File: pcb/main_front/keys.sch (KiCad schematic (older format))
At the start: 303 parts

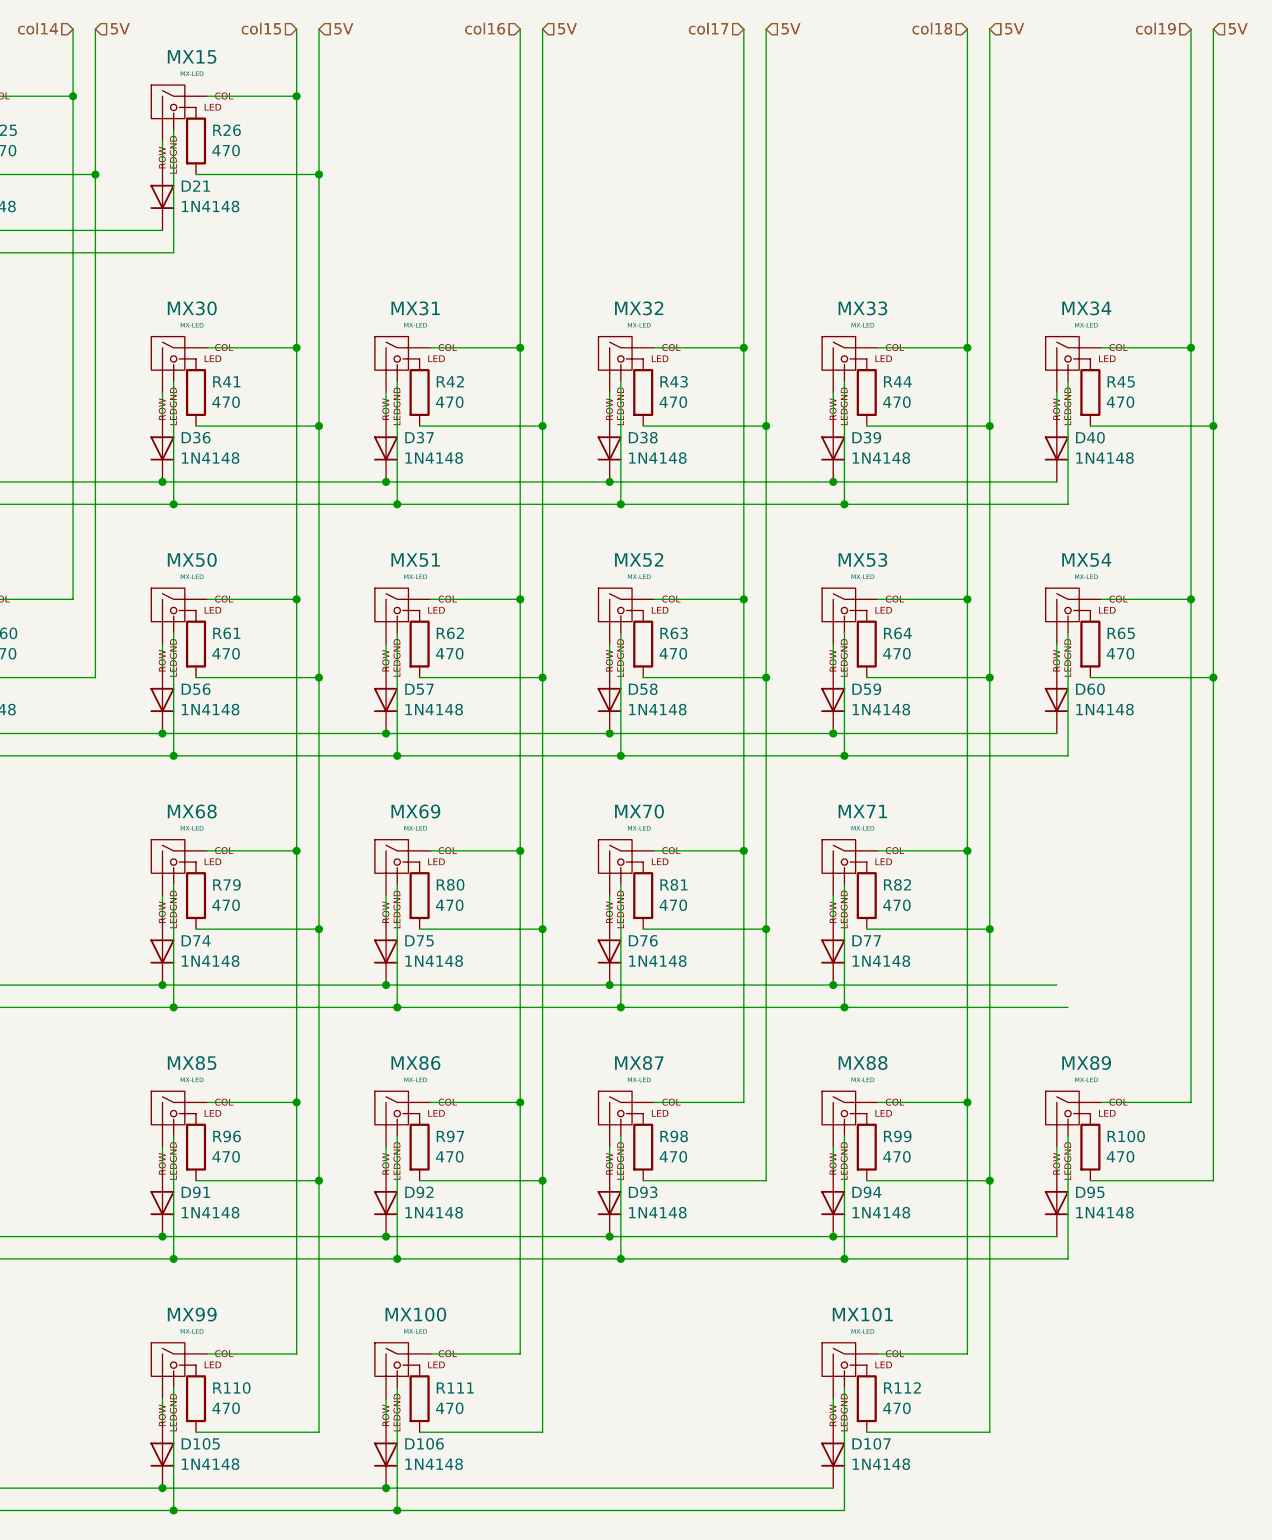
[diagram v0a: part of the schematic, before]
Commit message: Begin revised PCB layout
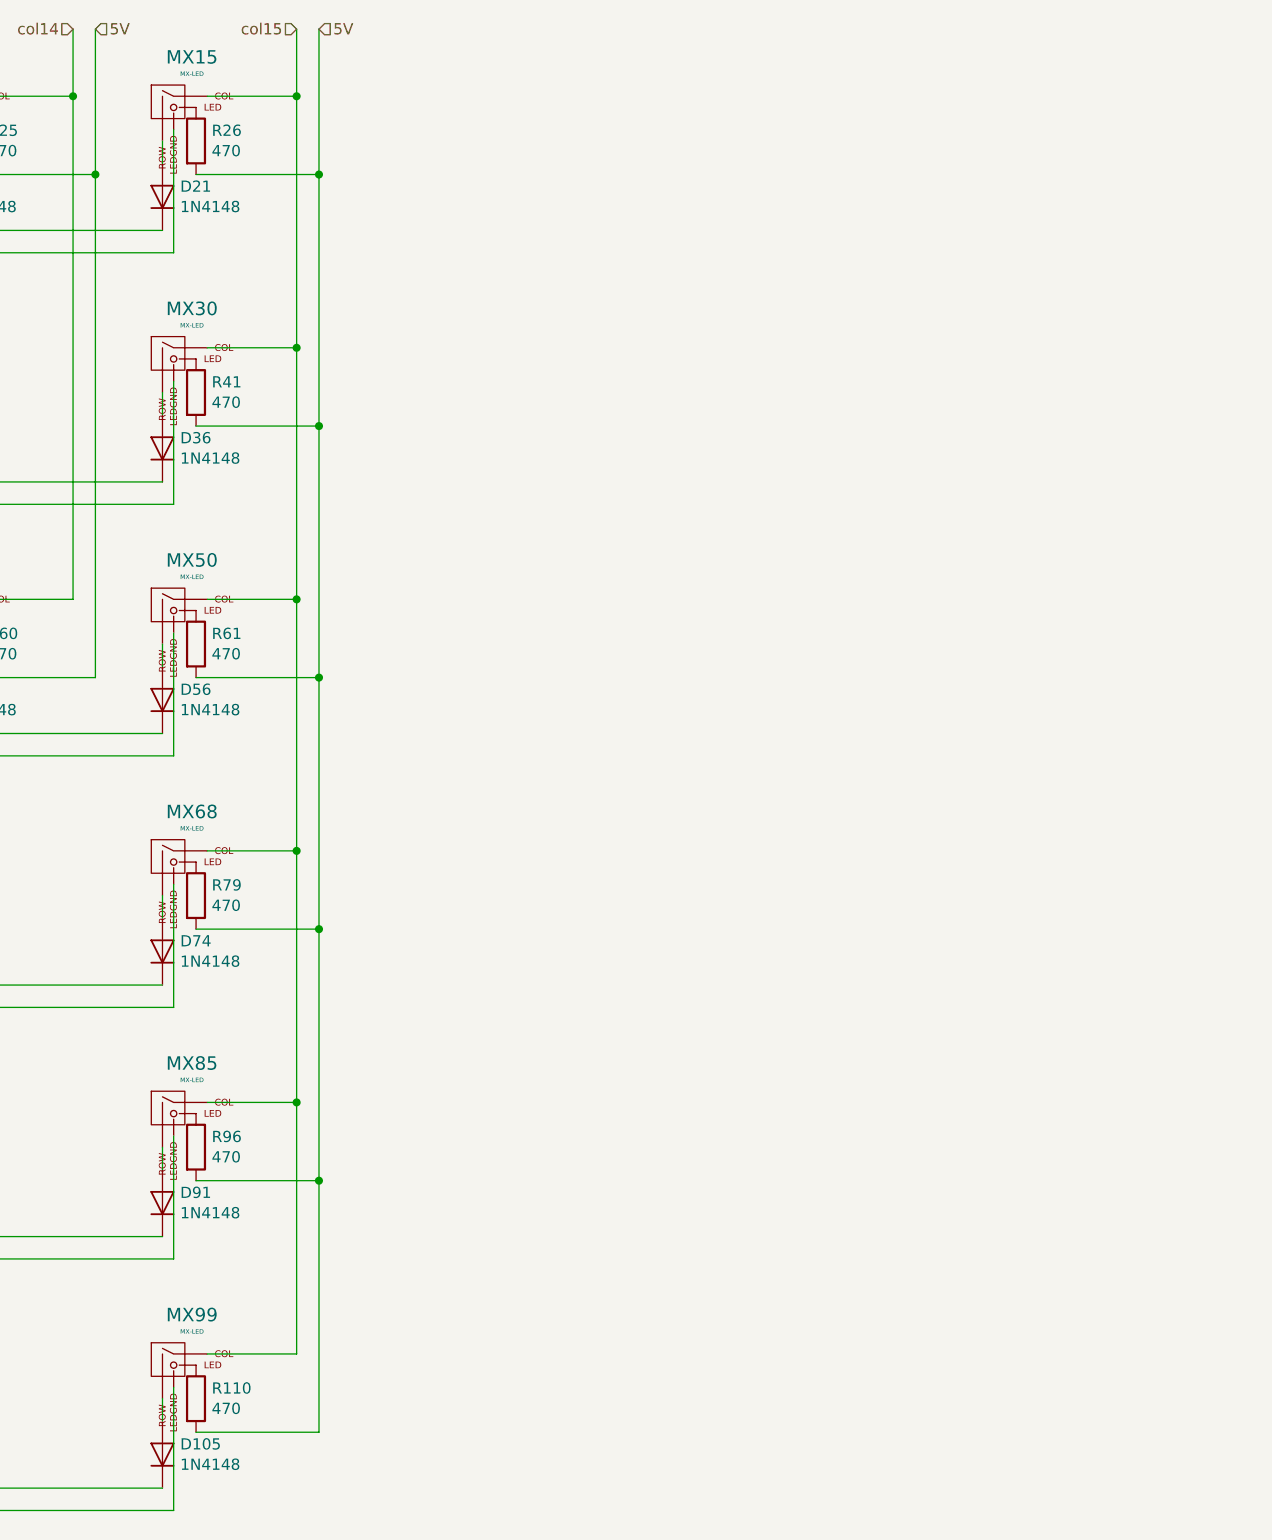
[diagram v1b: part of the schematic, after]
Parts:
- removed D106, D107, D37, D38, D39, D40, D57, D58, D59, D60, D75, D76, D77, D92, D93, D94, D95: 1N4148, Diode_THT:D_DO-35_SOD27_P7.62mm_Horizontal, symbol Device:D
- removed MX100: MX-LED, MX_Only:MXOnly-2U-ReversedStabilizers, symbol mx-led:MX-LED
- removed MX101, MX31, MX32, MX33, MX34, MX51, MX52, MX53, MX69, MX70, MX71, MX86, MX87, MX88: MX-LED, MX_Only:MXOnly-1U, symbol mx-led:MX-LED
- removed MX54, MX89: MX-LED, MX_Only:MXOnly-2U-ReversedVerticalStabilizers, symbol mx-led:MX-LED
- removed R100, R111, R112, R42, R43, R44, R45, R62, R63, R64, R65, R80, R81, R82, R97, R98, R99: 470, Resistor_THT:R_Axial_DIN0204_L3.6mm_D1.6mm_P7.62mm_Horizontal, symbol Device:R
